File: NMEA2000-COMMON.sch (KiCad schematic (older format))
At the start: 65 parts, among them J2 CAN, SW1 PRG, SW2 INSTANCE, SW3 BUS, U1 MCP2551-I-P, U101 74LS165, U2 TMR-2-2411, U3 74HCT595, U4 74HCT595, U5 Teensy_4.0

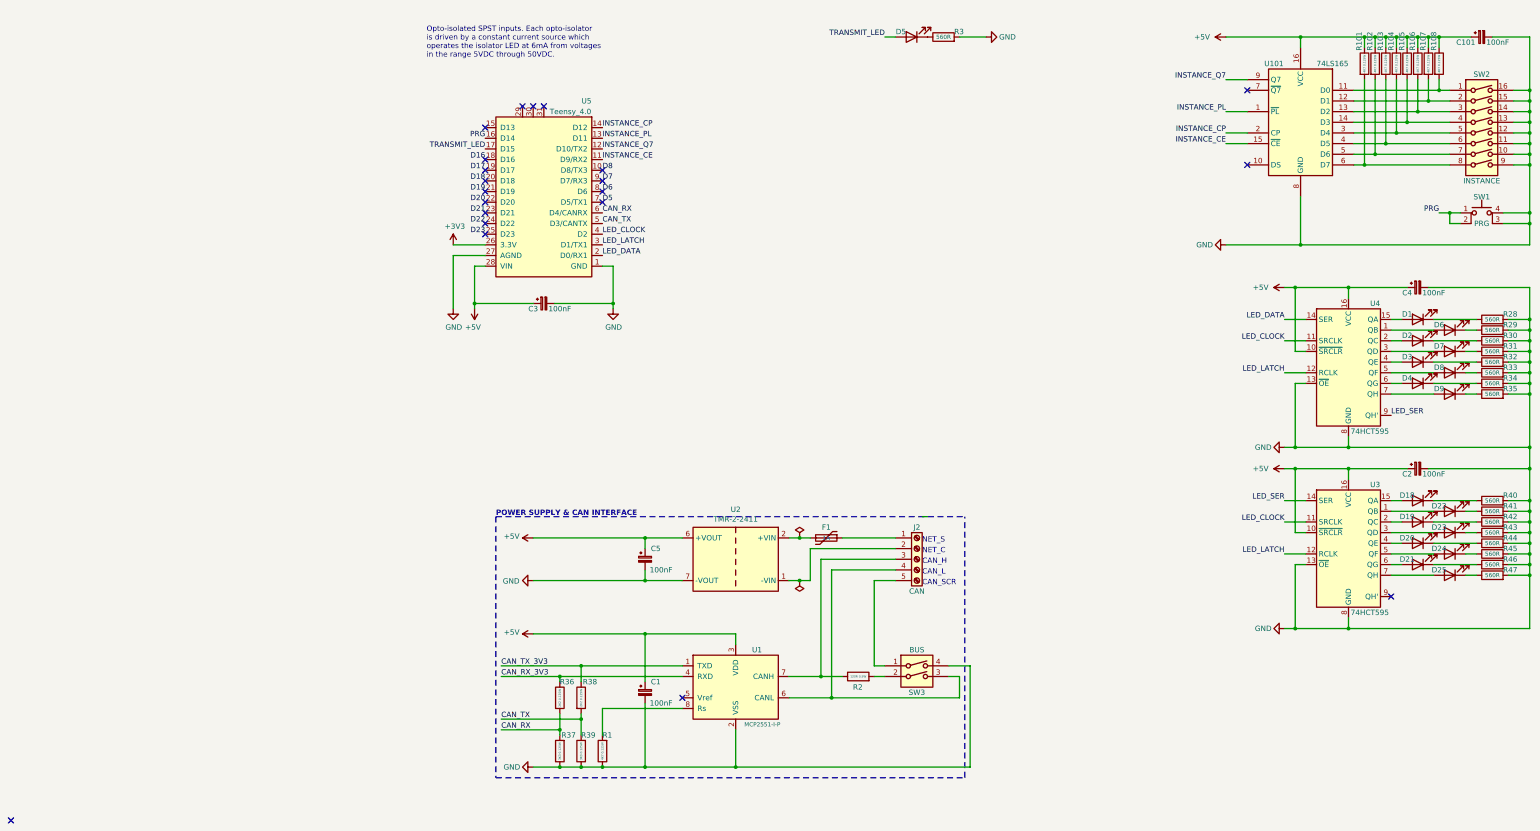
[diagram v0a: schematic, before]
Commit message: Tweak
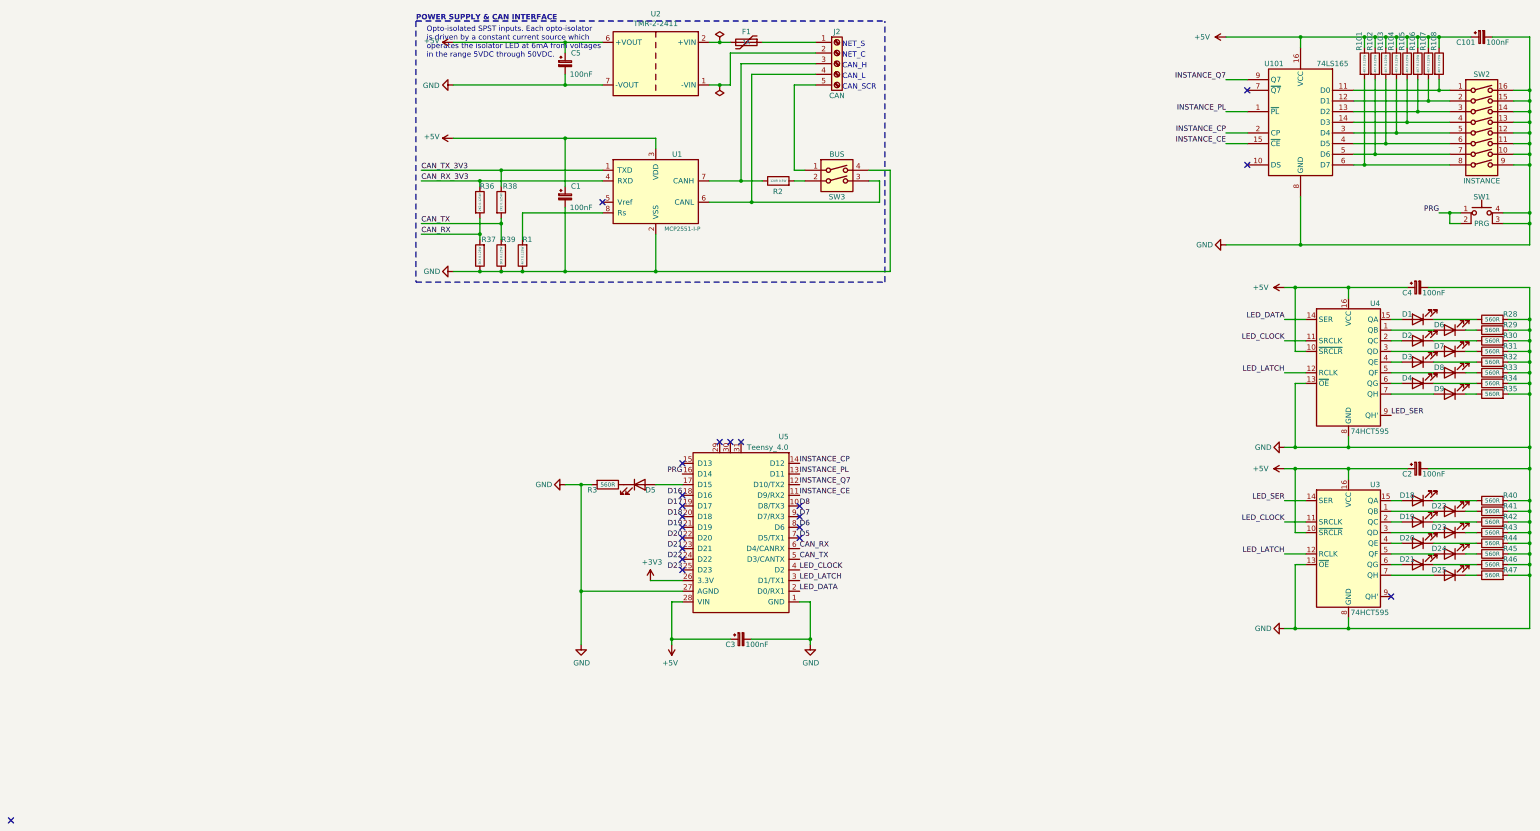
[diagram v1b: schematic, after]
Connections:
- net TRANSMIT_LED: no longer names the net of D5.2 (A), U5.17 (D15)
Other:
- moved on the sheet: C1, C3, C5, D5, F1, J2, R1, R2, R3, R36, R37, R38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
